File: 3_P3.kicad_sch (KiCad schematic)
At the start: 13 parts, among them J2 USB_B, J3 Expansion Header

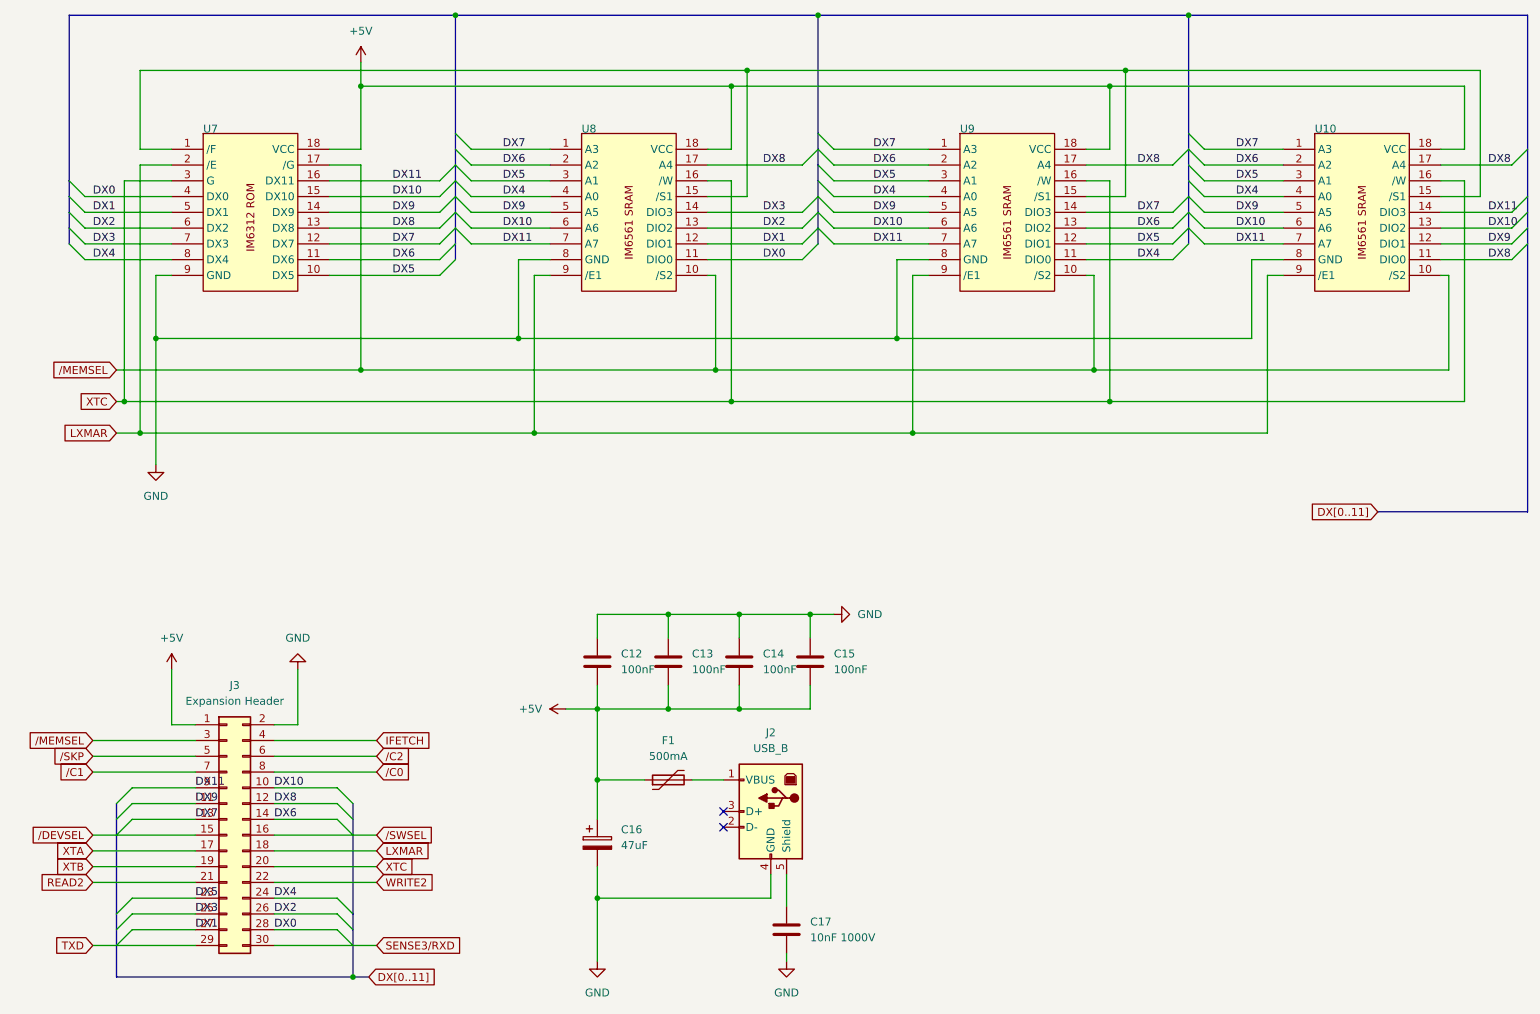
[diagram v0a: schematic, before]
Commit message: HID board finalizing
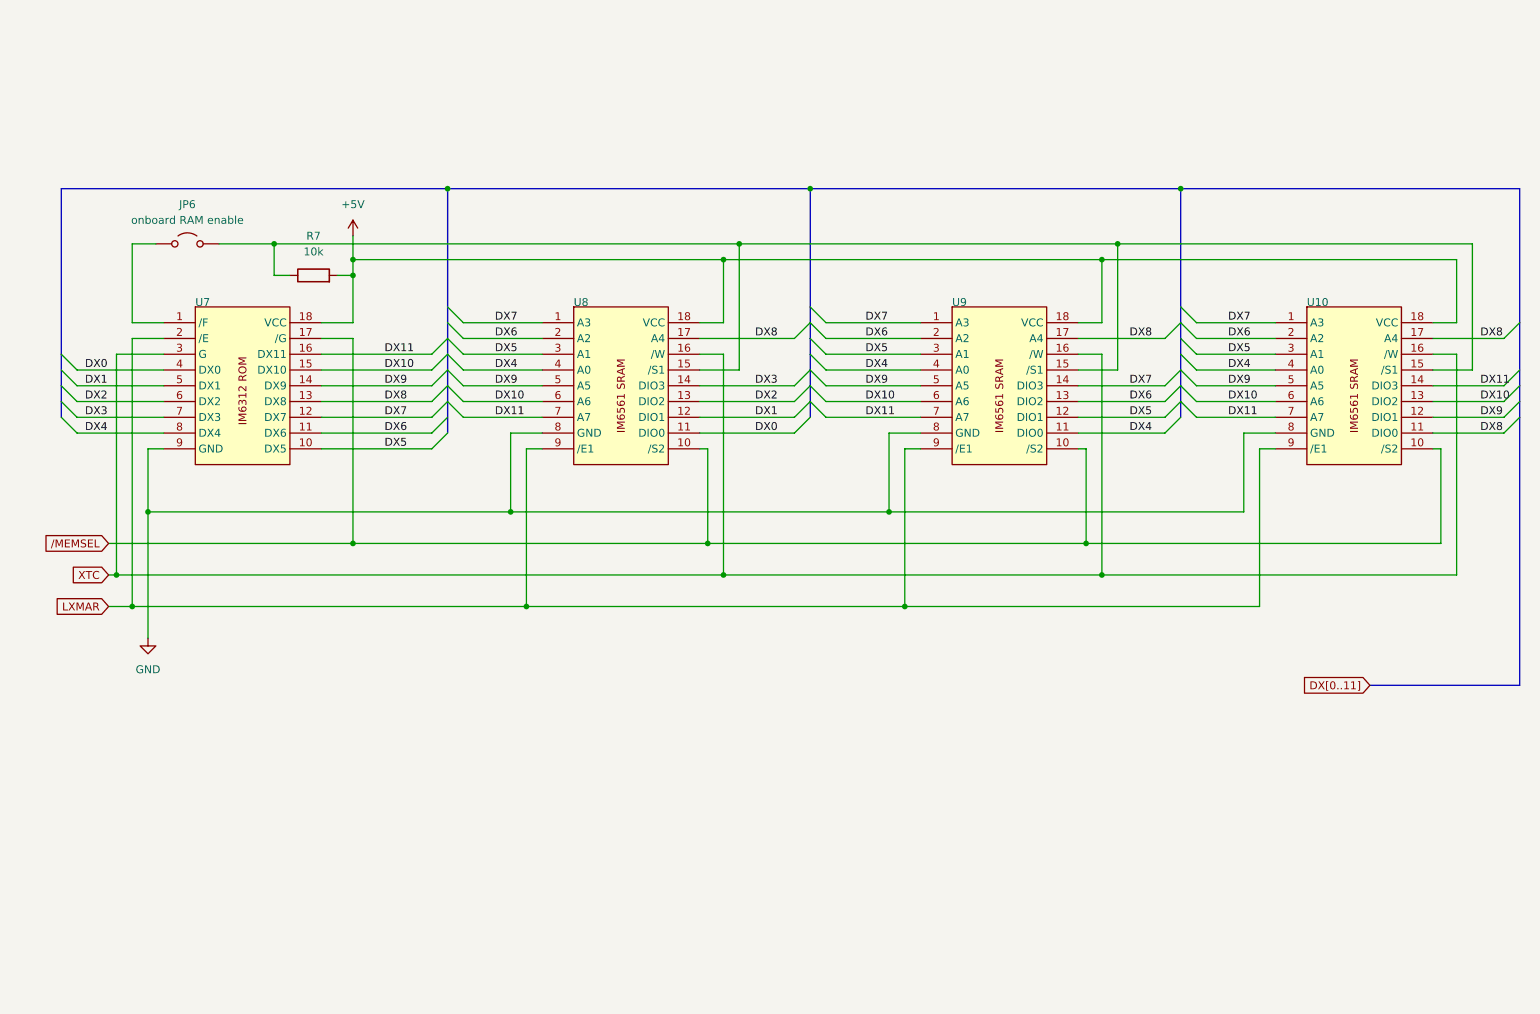
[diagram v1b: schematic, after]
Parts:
- removed C12, C13, C14, C15: 100nF, Capacitor_THT:C_Disc_D5.0mm_W2.5mm_P2.50mm, symbol Device:C
- removed C16: 47uF, Capacitor_THT:CP_Radial_D6.3mm_P2.50mm, symbol Device:C_Polarized
- removed C17: 10nF 1000V, Capacitor_THT:C_Disc_D5.0mm_W2.5mm_P2.50mm, symbol Device:C
- removed F1: 500mA, Capacitor_THT:C_Disc_D6.0mm_W2.5mm_P5.00mm, symbol Device:Polyfuse
- removed J2: USB_B, Connector_USB:USB_B_Lumberg_2411_02_Horizontal, symbol Connector:USB_B
- removed J3: Expansion Header, Connector_IDC:IDC-Header_2x15_P2.54mm_Vertical, symbol Connector_Generic:Conn_02x15_Odd_Even
- added JP6: onboard RAM enable, Connector_PinHeader_2.54mm:PinHeader_1x02_P2.54mm_Vertical, symbol Jumper:Jumper_2_Open
- added R7: 10k, Resistor_THT:R_Axial_DIN0207_L6.3mm_D2.5mm_P7.62mm_Horizontal, symbol Device:R
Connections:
- net +5V: now also R7.2
- net at U10.15 (/S1), U8.15 (/S1), U9.15 (/S1): now also JP6.2 (B), R7.1; no longer U7.1 (/F)
- new net: JP6.1 (A), U7.1 (/F)
- no-connect marks 2 -> 0
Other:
- moved on the sheet: U10, U7, U8, U9
